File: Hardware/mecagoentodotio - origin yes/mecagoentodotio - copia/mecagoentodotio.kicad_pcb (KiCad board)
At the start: 2 copper layers, 62.5 x 83 mm, 32 parts, among them J2 12V EN SERIE, J3 Screw_Terminal_01x02, J4 Screw_Terminal_01x02, J5 Screw_Terminal_01x02, J6 Screw_Terminal_01x02, SW3 SW_DPST_x2, SW4 SW_Push_Dual_x2, SW5 SW_Push_Dual_x2, U2 AMS1117-3.3, U3 AMS1117-5.0, U4 VTB6612_BREAKOUT, U5 ESP32-WROOM-32

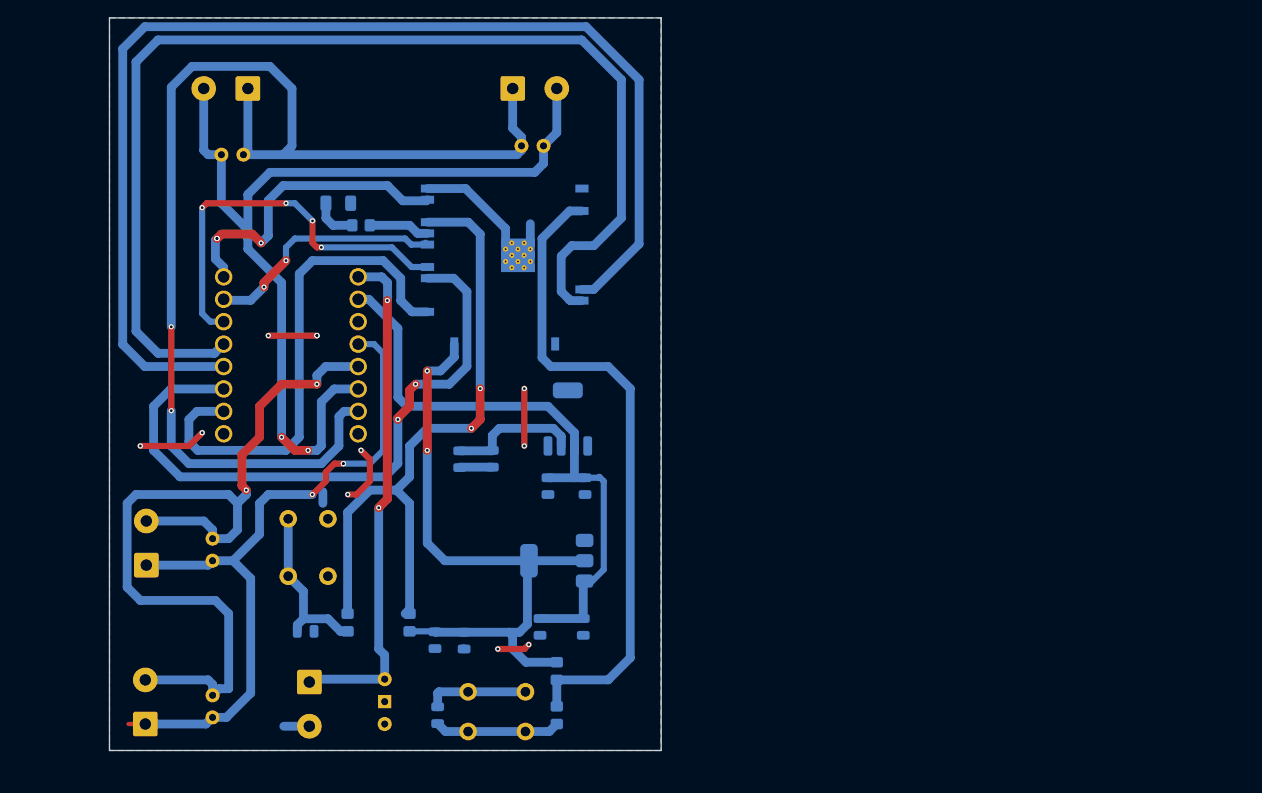
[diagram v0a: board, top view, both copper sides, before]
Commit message: 9/6 16:12
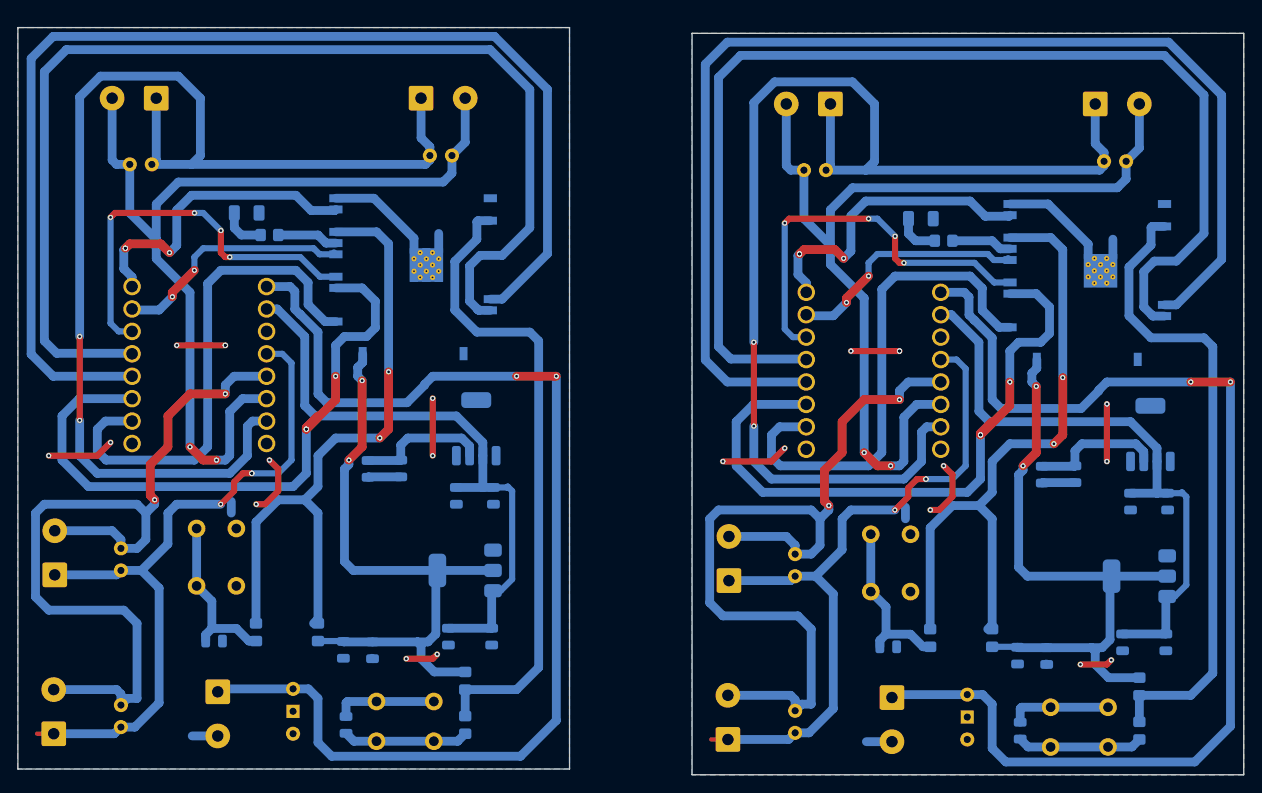
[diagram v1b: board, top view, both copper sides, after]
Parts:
- removed the C1 at (61.2, 170.5)
- removed the C10 at (92.9, 154.1)
- removed the C11 at (50.7, 180.2)
- removed the C12 at (50.7, 162.5)
- removed the C13 at (54.2, 116.5)
- removed the C14 at (85.7, 115.5)
- removed the C2 at (76.2, 180.0)
- removed the C3 at (87.8, 170.0)
- removed the C4 at (92.7, 170.0)
- removed the C5 at (78.7, 151.0)
- removed the C6 at (82.4, 150.9)
- removed the C7 at (79.2, 171.6)
- removed the C8 at (75.9, 171.5)
- removed the C9 at (88.7, 154.1)
- removed the D1 at (64.9, 122.0)
- removed the J2 at (61.6, 176.2)
- removed the J3 at (43.2, 163.0)
- removed the J4 at (43.1, 181.0)
- removed the J5 at (84.7, 109.0)
- removed the J6 at (54.7, 109.0)
- removed the R1 at (66.0, 169.5)
- removed the R2 at (89.7, 180.0)
- removed the R3 at (73.0, 169.5)
- removed the R4 at (89.7, 175.0)
- removed the R5 at (67.5, 124.5)
- removed the SW3 at (70.2, 178.5)
- removed the SW4 at (63.8, 164.2)
- removed the SW5 at (86.1, 177.3)
- removed the U2 at (89.7, 162.5)
- removed the U3 at (90.9, 146.4)
- removed the U4 at (59.6, 139.2)
- removed the U5 at (83.8, 128.6)
- added C1: C, Capacitor_SMD:C_0805_2012Metric, B.Cu at (127.2, 172.2)
- added C1: C, Capacitor_SMD:C_0805_2012Metric, B.Cu at (50.9, 171.6)
- added C10: 100nF, Capacitor_SMD:C_0805_2012Metric, B.Cu at (82.5, 155.2)
- added C10: 100nF, Capacitor_SMD:C_0805_2012Metric, B.Cu at (158.9, 155.8)
- added C11: 470uF, Capacitor_THT:C_Disc_D3.0mm_W1.6mm_P2.50mm, B.Cu at (116.7, 182.0)
- added C11: 470uF, Capacitor_THT:C_Disc_D3.0mm_W1.6mm_P2.50mm, B.Cu at (40.3, 181.3)
- added C12: 470uF, Capacitor_THT:C_Disc_D3.0mm_W1.6mm_P2.50mm, B.Cu at (116.7, 164.2)
- added C12: 470uF, Capacitor_THT:C_Disc_D3.0mm_W1.6mm_P2.50mm, B.Cu at (40.3, 163.6)
- added C13: 470uF, Capacitor_THT:C_Disc_D3.0mm_W1.6mm_P2.50mm, B.Cu at (120.2, 118.2)
- added C13: 470uF, Capacitor_THT:C_Disc_D3.0mm_W1.6mm_P2.50mm, B.Cu at (43.8, 117.6)
- added C14: 470uF, Capacitor_THT:C_Disc_D3.0mm_W1.6mm_P2.50mm, B.Cu at (151.7, 117.2)
- added C14: 470uF, Capacitor_THT:C_Disc_D3.0mm_W1.6mm_P2.50mm, B.Cu at (75.3, 116.6)
- added C2: C, Capacitor_SMD:C_0805_2012Metric, B.Cu at (142.2, 181.8)
- added C2: C, Capacitor_SMD:C_0805_2012Metric, B.Cu at (65.8, 181.1)
- added C3: 100n, Capacitor_SMD:C_0805_2012Metric, B.Cu at (77.4, 171.1)
- added C3: 100n, Capacitor_SMD:C_0805_2012Metric, B.Cu at (153.8, 171.8)
- added C4: 10u, Capacitor_SMD:C_0805_2012Metric, B.Cu at (158.7, 171.8)
- added C4: 10u, Capacitor_SMD:C_0805_2012Metric, B.Cu at (82.3, 171.1)
- added C5: 100u, Capacitor_SMD:C_0805_2012Metric, B.Cu at (68.3, 152.1)
- added C5: 100u, Capacitor_SMD:C_0805_2012Metric, B.Cu at (144.7, 152.8)
- added C6: 100nF, Capacitor_SMD:C_0805_2012Metric, B.Cu at (72.0, 152.1)
- added C6: 100nF, Capacitor_SMD:C_0805_2012Metric, B.Cu at (148.4, 152.7)
- added C7: 100n, Capacitor_SMD:C_0805_2012Metric, B.Cu at (145.2, 173.3)
- added C7: 100n, Capacitor_SMD:C_0805_2012Metric, B.Cu at (68.8, 172.7)
- added C8: 100n, Capacitor_SMD:C_0805_2012Metric, B.Cu at (65.5, 172.6)
- added C8: 100n, Capacitor_SMD:C_0805_2012Metric, B.Cu at (141.9, 173.2)
- added C9: 100u, Capacitor_SMD:C_0805_2012Metric, B.Cu at (78.3, 155.2)
- added C9: 100u, Capacitor_SMD:C_0805_2012Metric, B.Cu at (154.7, 155.8)
- added D1: LED, LED_SMD:LED_1206_3216Metric, B.Cu at (130.9, 123.8)
- added D1: LED, LED_SMD:LED_1206_3216Metric, B.Cu at (54.5, 123.1)
- added J2: 12V EN SERIE, TerminalBlock:TerminalBlock_MaiXu_MX126-5.0-02P_1x02_P5.00mm, B.Cu at (127.6, 178.0)
- added J2: 12V EN SERIE, TerminalBlock:TerminalBlock_MaiXu_MX126-5.0-02P_1x02_P5.00mm, B.Cu at (51.3, 177.3)
- added J3: Screw_Terminal_01x02, TerminalBlock:TerminalBlock_MaiXu_MX126-5.0-02P_1x02_P5.00mm, B.Cu at (109.2, 164.8)
- added J3: Screw_Terminal_01x02, TerminalBlock:TerminalBlock_MaiXu_MX126-5.0-02P_1x02_P5.00mm, B.Cu at (32.8, 164.1)
- added J4: Screw_Terminal_01x02, TerminalBlock:TerminalBlock_MaiXu_MX126-5.0-02P_1x02_P5.00mm, B.Cu at (109.1, 182.8)
- added J4: Screw_Terminal_01x02, TerminalBlock:TerminalBlock_MaiXu_MX126-5.0-02P_1x02_P5.00mm, B.Cu at (32.7, 182.1)
- added J5: Screw_Terminal_01x02, TerminalBlock:TerminalBlock_MaiXu_MX126-5.0-02P_1x02_P5.00mm, B.Cu at (74.3, 110.1)
- added J5: Screw_Terminal_01x02, TerminalBlock:TerminalBlock_MaiXu_MX126-5.0-02P_1x02_P5.00mm, B.Cu at (150.7, 110.8)
- added J6: Screw_Terminal_01x02, TerminalBlock:TerminalBlock_MaiXu_MX126-5.0-02P_1x02_P5.00mm, B.Cu at (44.3, 110.1)
- added J6: Screw_Terminal_01x02, TerminalBlock:TerminalBlock_MaiXu_MX126-5.0-02P_1x02_P5.00mm, B.Cu at (120.7, 110.8)
- added R1: 470, Resistor_SMD:R_0805_2012Metric_Pad1.20x1.40mm_HandSolder, B.Cu at (55.6, 170.6)
- added R1: 470, Resistor_SMD:R_0805_2012Metric_Pad1.20x1.40mm_HandSolder, B.Cu at (132.0, 171.2)
- added R2: 470, Resistor_SMD:R_0805_2012Metric_Pad1.20x1.40mm_HandSolder, B.Cu at (79.3, 181.1)
- added R2: 470, Resistor_SMD:R_0805_2012Metric_Pad1.20x1.40mm_HandSolder, B.Cu at (155.7, 181.8)
- added R3: 10K, Resistor_SMD:R_0805_2012Metric_Pad1.20x1.40mm_HandSolder, B.Cu at (62.6, 170.6)
- added R3: 10K, Resistor_SMD:R_0805_2012Metric_Pad1.20x1.40mm_HandSolder, B.Cu at (139.0, 171.2)
- added R4: 10K, Resistor_SMD:R_0805_2012Metric_Pad1.20x1.40mm_HandSolder, B.Cu at (79.3, 176.1)
- added R4: 10K, Resistor_SMD:R_0805_2012Metric_Pad1.20x1.40mm_HandSolder, B.Cu at (155.7, 176.8)
- added R5: 330, Resistor_SMD:R_0805_2012Metric_Pad1.20x1.40mm_HandSolder, B.Cu at (57.1, 125.6)
- added R5: 330, Resistor_SMD:R_0805_2012Metric_Pad1.20x1.40mm_HandSolder, B.Cu at (133.5, 126.2)
- added SW3: SW_DPST_x2, Button_Switch_THT:SW_Slide-03_Wuerth-WS-SLTV_10x2.5x6.4_P2.54mm, B.Cu at (59.8, 179.6)
- added SW3: SW_DPST_x2, Button_Switch_THT:SW_Slide-03_Wuerth-WS-SLTV_10x2.5x6.4_P2.54mm, B.Cu at (136.2, 180.2)
- added SW4: SW_Push_Dual_x2, Button_Switch_THT:SW_PUSH_6mm_H5mm, B.Cu at (53.4, 165.3)
- added SW4: SW_Push_Dual_x2, Button_Switch_THT:SW_PUSH_6mm_H5mm, B.Cu at (129.8, 166.0)
- added SW5: SW_Push_Dual_x2, Button_Switch_THT:SW_PUSH_6mm_H5mm, B.Cu at (152.1, 179.1)
- added SW5: SW_Push_Dual_x2, Button_Switch_THT:SW_PUSH_6mm_H5mm, B.Cu at (75.8, 178.4)
- added U2: AMS1117-3.3, Package_TO_SOT_SMD:SOT-223-3_TabPin2, B.Cu at (79.3, 163.6)
- added U2: AMS1117-3.3, Package_TO_SOT_SMD:SOT-223-3_TabPin2, B.Cu at (155.7, 164.2)
- added U3: AMS1117-5.0, Package_TO_SOT_SMD:SOT-223-5, B.Cu at (80.5, 147.6)
- added U3: AMS1117-5.0, Package_TO_SOT_SMD:SOT-223-5, B.Cu at (156.9, 148.2)
- added U4: VTB6612_BREAKOUT, huellasdelcole:tb6612fng, B.Cu at (49.2, 140.3)
- added U4: VTB6612_BREAKOUT, huellasdelcole:tb6612fng, B.Cu at (125.6, 141.0)
- added U5: ESP32-WROOM-32, RF_Module:ESP32-WROOM-32U, B.Cu at (149.8, 130.3)
- added U5: ESP32-WROOM-32, RF_Module:ESP32-WROOM-32U, B.Cu at (73.4, 129.7)
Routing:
- net 7,5V: track 57.9 -> 260.2 mm, vias 2 -> 4
- net B1: track 137.5 -> 275.1 mm, vias 2 -> 4
- net BIN1: track 135.2 -> 270.4 mm
- net STBY: track 130.9 -> 260.0 mm
- net B2: track 108.2 -> 216.4 mm, vias 2 -> 4
- net A2: track 96.5 -> 193.0 mm, vias 2 -> 4
- net A1: track 80.9 -> 161.8 mm, vias 3 -> 6
- net BIN2: track 73.4 -> 149.3 mm, vias 2 -> 6
- net 1O1: track 75.3 -> 150.5 mm, vias 2 -> 4
- net EN: track 73.6 -> 145.8 mm
- net 3.3V: track 72.2 -> 141.7 mm, vias 2 -> 4
- net VCC: track 68.9 -> 137.9 mm
- net GND: track 64.5 -> 128.9 mm, vias 11 -> 22
- net PWMB: track 57.9 -> 115.7 mm
- net AIN1: track 45.0 -> 90.0 mm, vias 4 -> 8
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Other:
- board size 62.5 x 83 mm -> 138.9 x 84.7 mm
